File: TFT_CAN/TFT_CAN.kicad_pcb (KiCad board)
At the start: 2 copper layers, 94 x 51 mm, 9 parts, among them J1 Conn_01x20, J2 Conn_01x20, SW1 Conn_01x02, SW2 Conn_01x02, U1 Teensy3.2

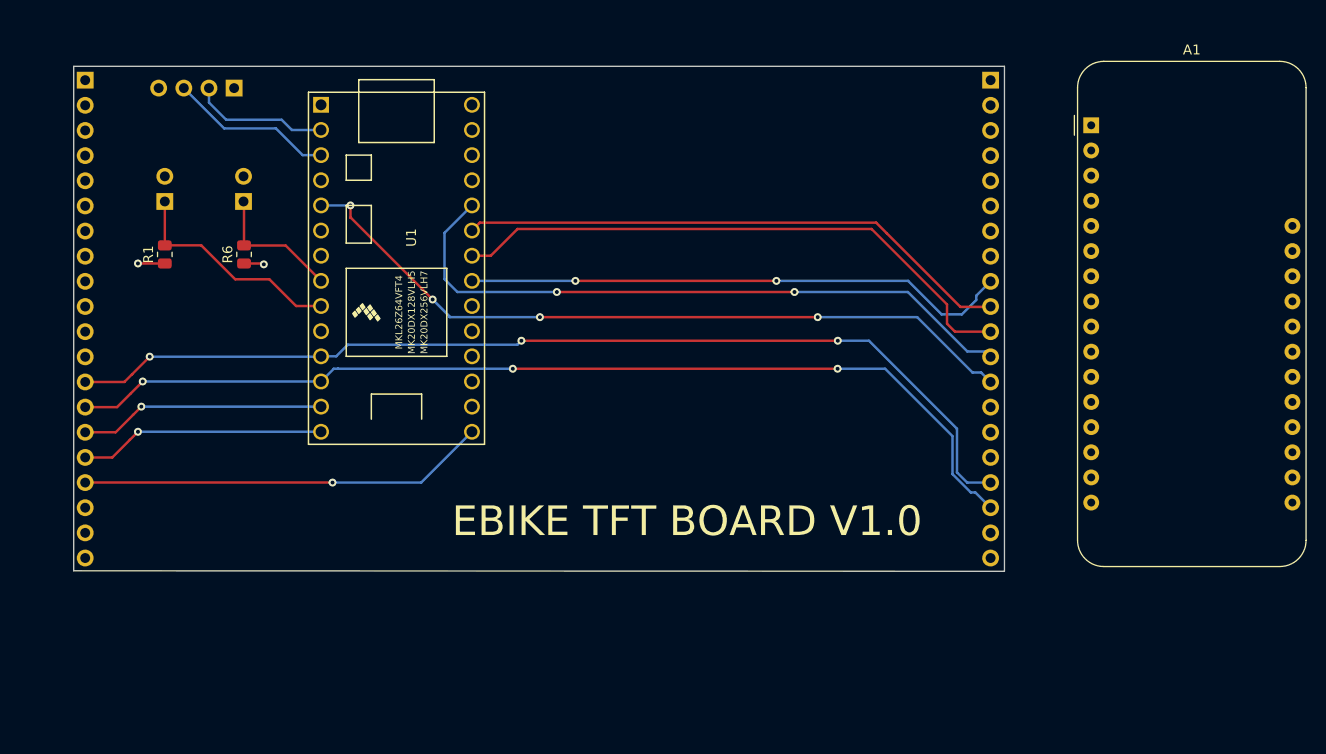
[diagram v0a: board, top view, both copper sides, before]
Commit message: finished layout
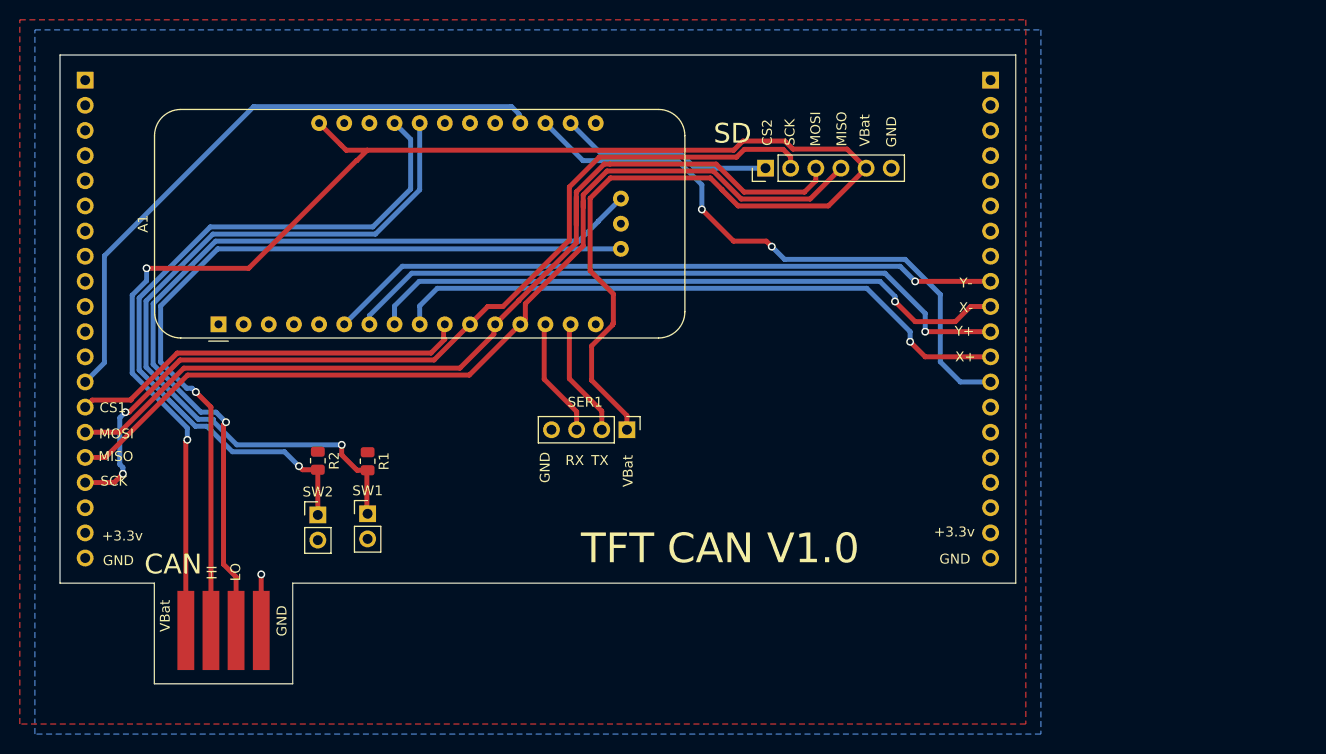
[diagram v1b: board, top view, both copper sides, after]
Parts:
- removed R6: 10k, Resistor_SMD:R_0805_2012Metric
- removed U1: Teensy3.2, teensy:Teensy32
- added CAN1: Conn_01x04, Connector_PinHeader_2.54mm:my_4_tab_edge, F.Cu at (35.6, 81.0)
- added J3: Conn_01x06, Connector_PinHeader_2.54mm:PinHeader_1x06_P2.54mm_Vertical, F.Cu at (94.1, 34.3)
- added R2: 10k, Resistor_SMD:R_0805_2012Metric, F.Cu at (48.9, 63.8)
- A1: footprint Module:Adafruit_Feather -> Module:Adafruit_Feather_M4_CAN
- SER1, SW1, SW2: moved to F.Cu
- moved A1 90.4 mm to (38.9, 50.1), turned to 90 degrees
- moved SER1 52.6 mm to (80.1, 60.7), turned to -90 degrees
- moved SW2 35.2 mm to (48.9, 69.3)
- moved SW1 33.9 mm to (53.9, 69.2)
- moved R1 29.3 mm to (53.9, 63.9), turned to -90 degrees
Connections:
- A1 pad 10: unconnected-(A1-Pad10) -> CS1
- A1 pad 11: unconnected-(A1-Pad11) -> SCK
- A1 pad 12: unconnected-(A1-Pad12) -> MOSI
- A1 pad 13: unconnected-(A1-Pad13) -> MISO
- A1 pad 14: unconnected-(A1-Pad14) -> RX
- A1 pad 15: unconnected-(A1-Pad15) -> TX
- A1 pad 18: unconnected-(A1-Pad18) -> CS2
- A1 pad 19: unconnected-(A1-Pad19) -> BK_LGHT
- A1 pad 2: unconnected-(A1-Pad2) -> +3.3v
- A1 pad 20: unconnected-(A1-Pad20) -> D/C
- A1 pad 24: unconnected-(A1-Pad24) -> PB1_IN
- A1 pad 25: unconnected-(A1-Pad25) -> PB2_IN
- A1 pad 28: unconnected-(A1-Pad28) -> VBat
- A1 pad 4: unconnected-(A1-Pad4) -> GND
- A1 pad 6: unconnected-(A1-Pad6) -> Y-
- A1 pad 7: unconnected-(A1-Pad7) -> Y+
- A1 pad 8: unconnected-(A1-Pad8) -> X-
- A1 pad 9: unconnected-(A1-Pad9) -> X+
- J1 pad 13: CD -> D/C
- J1 pad 14: CS -> CS1
- J2 pad 13: BRIGHTNESS -> BK_LGHT
- J2 pad 15: RD -> unconnected-(J2-Pad15)
- J2 pad 16: WR -> unconnected-(J2-Pad16)
- J2 pad 17: CD -> unconnected-(J2-Pad17)
- J2 pad 18: CS -> unconnected-(J2-Pad18)
- R1 pad 2: PB2_IN -> PB1_IN
- SER1 pad 1: +3.3v -> VBat
- SER1 pad 2: Tx-BESC -> TX
- SER1 pad 3: Rx-BESC -> RX
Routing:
- net VBat: track 0.00 -> 182.6 mm, vias 0 -> 2
- net CD: track 101.8 -> 0.00 mm, vias 3 -> 0
- net CS: track 101.3 -> 0.00 mm, vias 3 -> 0
- net CAN_LO: track 0.00 -> 88.9 mm, vias 0 -> 1
- net CAN_HI: track 0.00 -> 86.3 mm, vias 0 -> 1
- net BRIGHTNESS: track 75.8 -> 0.00 mm, vias 4 -> 0
- net MISO: track 24.9 -> 95.1 mm, vias 1 -> 0
- net MOSI: track 24.9 -> 94.0 mm, vias 1 -> 0
- net PB1_IN: track 13.7 -> 77.5 mm, vias 0 -> 1
- net D/C: track 0.00 -> 63.0 mm
- net BK_LGHT: track 0.00 -> 61.2 mm, vias 0 -> 2
- net SCK: track 41.2 -> 93.4 mm, vias 1 -> 2
- net PB2_IN: track 22.8 -> 73.2 mm, vias 0 -> 1
- net CS1: track 0.00 -> 40.7 mm
- net CS2: track 0.00 -> 21.6 mm
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- added copper zone on F.Cu, net +3.3v
- added copper zone on B.Cu, net GND
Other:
- board size 94 x 51 mm -> 96.5 x 63.5 mm
- board text added: "+3.3v"
- board text added: "CAN"
- board text added: "CS1"
- board text added: "CS2"
- board text added: "GND"
- board text added: "HI"
- board text added: "LO"
- board text added: "MISO"
- board text added: "MOSI"
- board text added: "RX"
- board text added: "SCK"
- board text added: "SD"
- board text added: "TFT CAN V1.0"
- board text added: "TX"
- board text added: "VBat"
- board text added: "X+"
- board text added: "X-"
- board text added: "Y+"
- board text added: "Y-"
- board text removed: "EBIKE TFT BOARD V1.0"
